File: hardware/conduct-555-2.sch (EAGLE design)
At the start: 15 parts, among them J2 AYZ0202

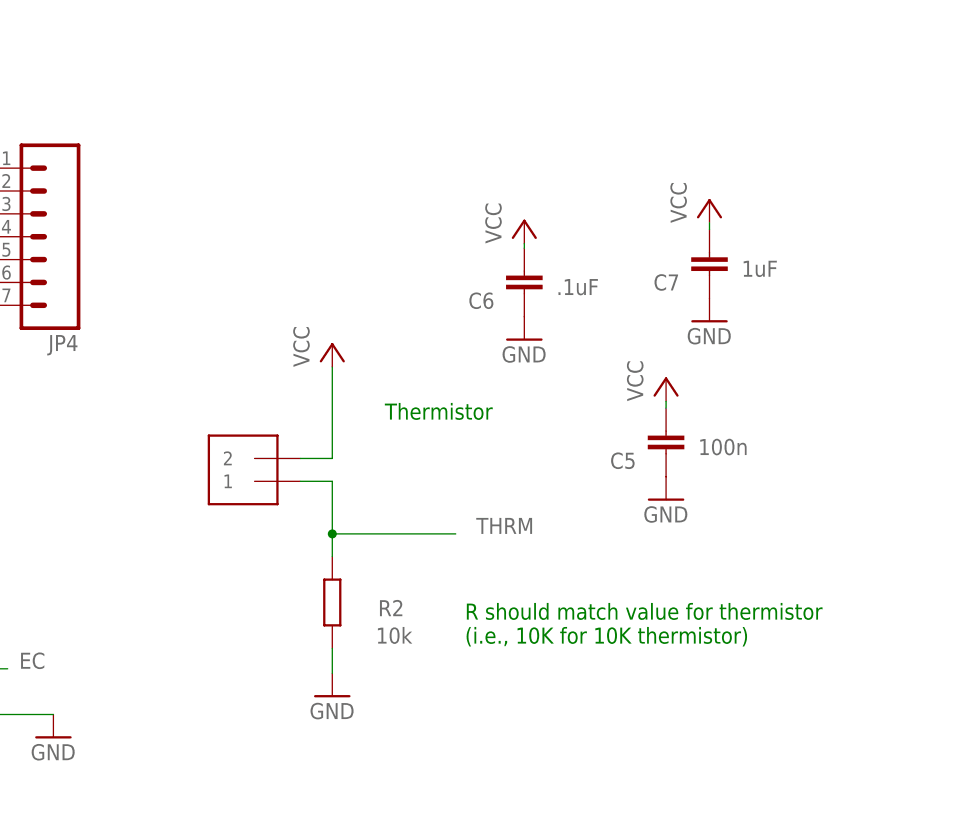
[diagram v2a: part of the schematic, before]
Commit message: update
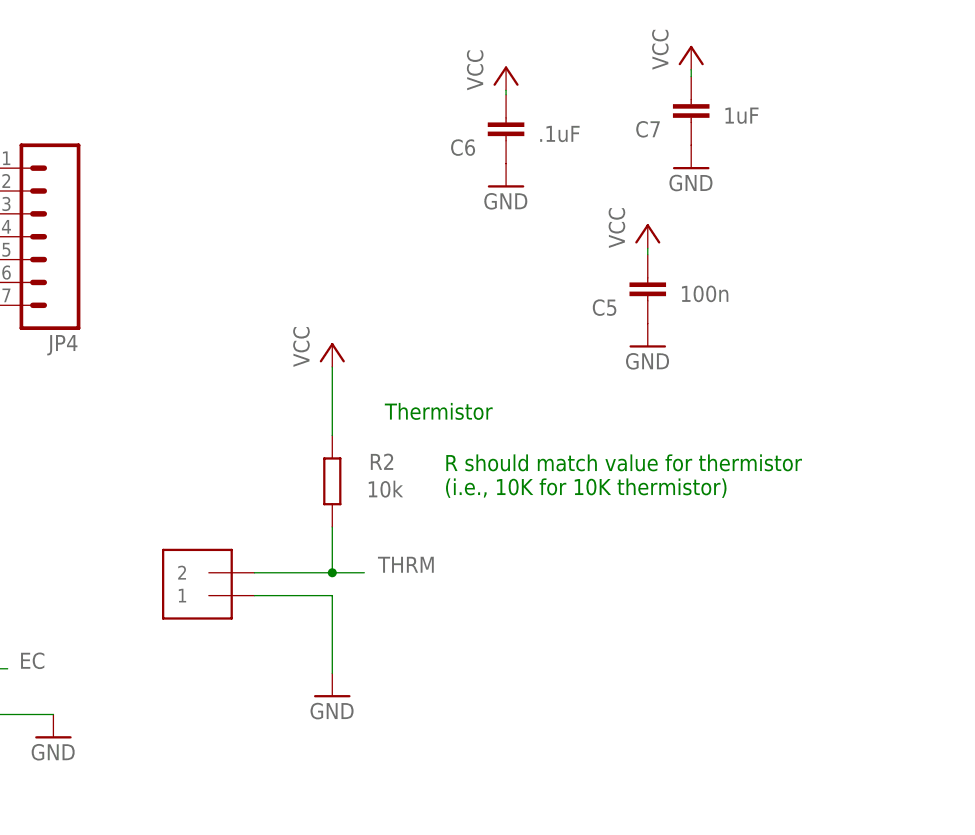
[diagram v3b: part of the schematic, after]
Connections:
- net GND: now also THRM.1; no longer R2.1
- net THRM: now also R2.1, THRM.2; no longer R2.2, THRM.1
- net VCC: now also R2.2; no longer THRM.2
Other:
- moved on the sheet: C5, C6, C7, R2
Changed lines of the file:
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@@
 <setting verticaltext="up"/>
 </settings>
-<grid distance="0.1" unitdist="inch" unit="inch" style="lines" multiple="1" display="no" altdistance="0.01" altunitdist="inch" altunit="inch"/>
+<grid distance="0.01" unitdist="inch" unit="inch" style="lines" multiple="1" display="no" altdistance="0.01" altunitdist="inch" altunit="inch"/>
 <layers>
 <layer number="1" name="Top" color="4" fill="1" visible="no" active="no"/>
@@
 <plain>
 <text x="165.862" y="85.09" size="1.778" layer="91">Thermistor</text>
-<text x="174.752" y="60.198" size="1.778" layer="91">R should match value for thermistor
+<text x="172.466" y="76.708" size="1.778" layer="91">R should match value for thermistor
 (i.e., 10K for 10K thermistor)</text>
 </plain>
@@
 <attribute name="VALUE" x="66.04" y="46.99" size="1.778" layer="96"/>
 </instance>
-<instance part="THRM" gate="G$1" x="151.384" y="80.772" rot="R180"/>
+<instance part="THRM" gate="G$1" x="146.304" y="68.072" rot="R180"/>
 <instance part="P+3" gate="VCC" x="66.04" y="42.672" rot="R90"/>
 <instance part="P+5" gate="VCC" x="160.02" y="93.472"/>
-<instance part="R2" gate="G$1" x="160.02" y="64.77" smashed="yes" rot="R90">
-<attribute name="NAME" x="165.1" y="63.246" size="1.778" layer="95"/>
-<attribute name="VALUE" x="164.846" y="60.198" size="1.778" layer="96"/>
+<instance part="R2" gate="G$1" x="160.02" y="78.232" smashed="yes" rot="R90">
+<attribute name="NAME" x="164.084" y="79.502" size="1.778" layer="95"/>
+<attribute name="VALUE" x="163.83" y="76.454" size="1.778" layer="96"/>
 </instance>
 <instance part="GND2" gate="1" x="160.02" y="54.356"/>
@@
 <instance part="EC" gate="G$1" x="81.534" y="80.772" rot="R90"/>
 <instance part="P+1" gate="VCC" x="108.458" y="97.79" rot="R90"/>
-<instance part="C5" gate="G$1" x="197.104" y="81.28" smashed="yes" rot="R180">
-<attribute name="NAME" x="193.802" y="81.407" size="1.778" layer="95" rot="R180"/>
-<attribute name="VALUE" x="200.66" y="81.153" size="1.778" layer="96"/>
-</instance>
-<instance part="GND3" gate="1" x="197.104" y="76.2"/>
-<instance part="P+6" gate="VCC" x="197.104" y="89.662"/>
-<instance part="C6" gate="G$1" x="181.356" y="99.06" smashed="yes" rot="R180">
-<attribute name="NAME" x="178.054" y="99.187" size="1.778" layer="95" rot="R180"/>
-<attribute name="VALUE" x="184.912" y="98.933" size="1.778" layer="96"/>
-</instance>
-<instance part="GND5" gate="1" x="181.356" y="93.98"/>
-<instance part="P+7" gate="VCC" x="181.356" y="107.188"/>
-<instance part="C7" gate="G$1" x="201.93" y="101.092" smashed="yes" rot="R180">
-<attribute name="NAME" x="198.628" y="101.219" size="1.778" layer="95" rot="R180"/>
-<attribute name="VALUE" x="205.486" y="100.965" size="1.778" layer="96"/>
-</instance>
-<instance part="GND6" gate="1" x="201.93" y="96.012"/>
-<instance part="P+8" gate="VCC" x="201.93" y="109.474"/>
+<instance part="C5" gate="G$1" x="195.072" y="98.298" smashed="yes" rot="R180">
+<attribute name="NAME" x="191.77" y="98.425" size="1.778" layer="95" rot="R180"/>
+<attribute name="VALUE" x="198.628" y="98.171" size="1.778" layer="96"/>
+</instance>
+<instance part="GND3" gate="1" x="195.072" y="93.218"/>
+<instance part="P+6" gate="VCC" x="195.072" y="106.68"/>
+<instance part="C6" gate="G$1" x="179.324" y="116.078" smashed="yes" rot="R180">
+<attribute name="NAME" x="176.022" y="116.205" size="1.778" layer="95" rot="R180"/>
+<attribute name="VALUE" x="182.88" y="115.951" size="1.778" layer="96"/>
+</instance>
+<instance part="GND5" gate="1" x="179.324" y="110.998"/>
+<instance part="P+7" gate="VCC" x="179.324" y="124.206"/>
+<instance part="C7" gate="G$1" x="199.898" y="118.11" smashed="yes" rot="R180">
+<attribute name="NAME" x="196.596" y="118.237" size="1.778" layer="95" rot="R180"/>
+<attribute name="VALUE" x="203.454" y="117.983" size="1.778" layer="96"/>
+</instance>
+<instance part="GND6" gate="1" x="199.898" y="113.03"/>
+<instance part="P+8" gate="VCC" x="199.898" y="126.492"/>
 <instance part="GND7" gate="1" x="108.966" y="115.57" rot="R180"/>
 <instance part="GND8" gate="1" x="64.262" y="99.06"/>
@@
 </segment>
 <segment>
-<pinref part="R2" gate="G$1" pin="1"/>
-<wire x1="160.02" y1="59.69" x2="160.02" y2="56.896" width="0.1524" layer="91"/>
-<pinref part="GND2" gate="1" pin="GND"/>
-</segment>
-<segment>
 <wire x1="121.666" y1="113.03" x2="108.966" y2="113.03" width="0.1524" layer="91"/>
 <pinref part="JP4" gate="G$1" pin="1"/>
@@
 <pinref part="JP2" gate="G$1" pin="1"/>
 <pinref part="GND8" gate="1" pin="GND"/>
+</segment>
+<segment>
+<pinref part="GND2" gate="1" pin="GND"/>
+<wire x1="160.02" y1="56.896" x2="160.02" y2="65.532" width="0.1524" layer="91"/>
+<pinref part="THRM" gate="G$1" pin="1"/>
+<wire x1="160.02" y1="65.532" x2="151.384" y2="65.532" width="0.1524" layer="91"/>
 </segment>
 </net>
@@
 <segment>
 <pinref part="P+5" gate="VCC" pin="VCC"/>
-<pinref part="THRM" gate="G$1" pin="2"/>
-<wire x1="156.464" y1="80.772" x2="160.02" y2="80.772" width="0.1524" layer="91"/>
-<wire x1="160.02" y1="80.772" x2="160.02" y2="90.932" width="0.1524" layer="91"/>
+<wire x1="160.02" y1="83.312" x2="160.02" y2="90.932" width="0.1524" layer="91"/>
+<pinref part="R2" gate="G$1" pin="2"/>
 </segment>
 <segment>
@@
 <pinref part="C5" gate="G$1" pin="2"/>
 <pinref part="P+6" gate="VCC" pin="VCC"/>
-<wire x1="197.104" y1="87.122" x2="197.104" y2="86.36" width="0.1524" layer="91"/>
+<wire x1="195.072" y1="104.14" x2="195.072" y2="103.378" width="0.1524" layer="91"/>
 </segment>
 <segment>
 <pinref part="C6" gate="G$1" pin="2"/>
 <pinref part="P+7" gate="VCC" pin="VCC"/>
-<wire x1="181.356" y1="104.648" x2="181.356" y2="104.14" width="0.1524" layer="91"/>
+<wire x1="179.324" y1="121.666" x2="179.324" y2="121.158" width="0.1524" layer="91"/>
 </segment>
 <segment>
 <pinref part="C7" gate="G$1" pin="2"/>
 <pinref part="P+8" gate="VCC" pin="VCC"/>
-<wire x1="201.93" y1="106.934" x2="201.93" y2="106.172" width="0.1524" layer="91"/>
+<wire x1="199.898" y1="123.952" x2="199.898" y2="123.19" width="0.1524" layer="91"/>
 </segment>
 </net>
@@
 <net name="THRM" class="0">
 <segment>
-<pinref part="THRM" gate="G$1" pin="1"/>
-<wire x1="156.464" y1="78.232" x2="160.02" y2="78.232" width="0.1524" layer="91"/>
-<wire x1="160.02" y1="78.232" x2="160.02" y2="72.39" width="0.1524" layer="91"/>
-<pinref part="R2" gate="G$1" pin="2"/>
-<wire x1="160.02" y1="72.39" x2="160.02" y2="69.85" width="0.1524" layer="91"/>
-<wire x1="160.02" y1="72.39" x2="173.736" y2="72.39" width="0.1524" layer="91"/>
-<label x="176.022" y="72.39" size="1.778" layer="95"/>
-<junction x="160.02" y="72.39"/>
-</segment>
-<segment>
 <wire x1="121.666" y1="110.49" x2="109.982" y2="110.49" width="0.1524" layer="91"/>
 <label x="104.902" y="110.49" size="1.778" layer="95"/>
 <pinref part="JP4" gate="G$1" pin="2"/>
 </segment>
-</net>
+<segment>
+<pinref part="THRM" gate="G$1" pin="2"/>
+<pinref part="R2" gate="G$1" pin="1"/>
+<wire x1="151.384" y1="68.072" x2="160.02" y2="68.072" width="0.1524" layer="91"/>
+<wire x1="160.02" y1="68.072" x2="160.02" y2="73.152" width="0.1524" layer="91"/>
+<wire x1="160.02" y1="68.072" x2="163.576" y2="68.072" width="0.1524" layer="91"/>
+<label x="165.1" y="68.072" size="1.778" layer="95"/>
+<junction x="160.02" y="68.072"/>
+</segment>
+</net>
